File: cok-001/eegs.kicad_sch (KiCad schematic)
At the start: 54 parts, among them U7005 LM75B

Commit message: switching regulator
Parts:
- R7044, R7045: footprint Resistor_SMD:R_0603_1608Metric -> Resistor_SMD:R_0402_1005Metric
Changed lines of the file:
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@@
 			)
 		)
-		(property "Footprint" "Resistor_SMD:R_0603_1608Metric"
+		(property "Footprint" "Resistor_SMD:R_0402_1005Metric"
 			(at 555.244 141.224 90)
 			(effects
@@
 			)
 		)
-		(property "Footprint" "Resistor_SMD:R_0603_1608Metric"
+		(property "Footprint" "Resistor_SMD:R_0402_1005Metric"
 			(at 555.244 138.684 90)
 			(effects

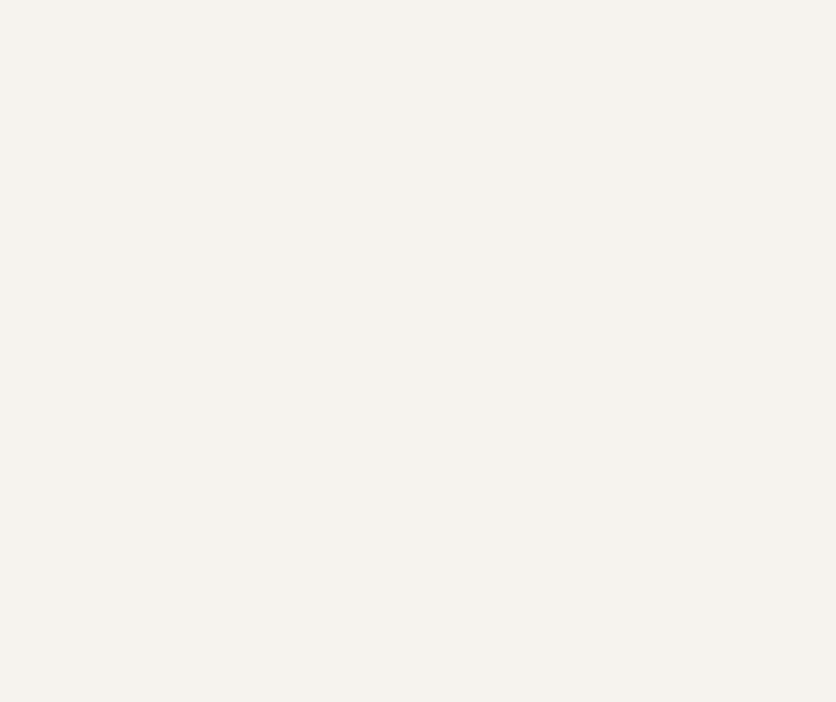
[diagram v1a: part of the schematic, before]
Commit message: temp sensor and clock
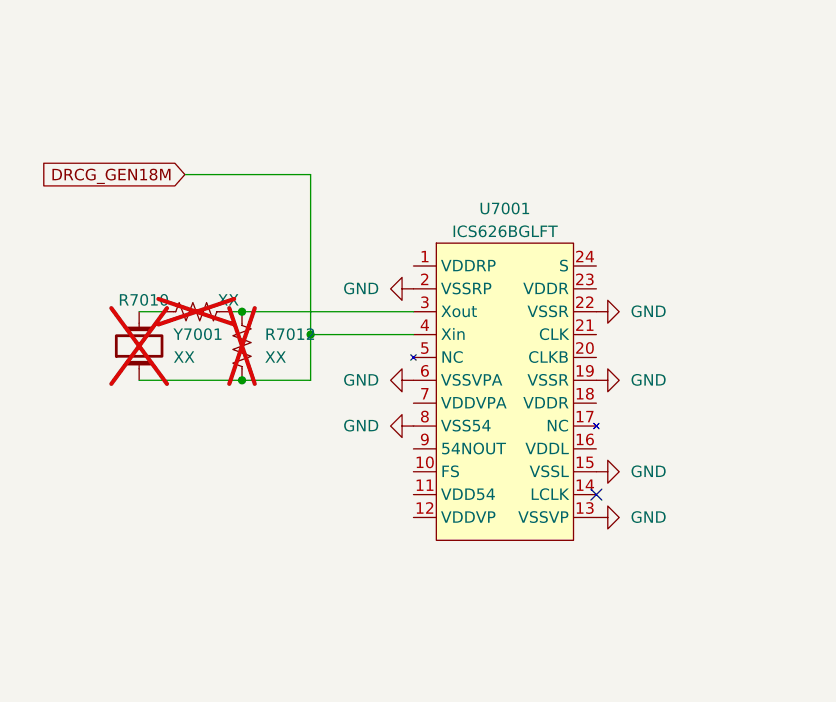
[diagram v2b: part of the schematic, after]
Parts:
- added R7010, R7012: XX, Resistor_SMD:R_0402_1005Metric, symbol Device:R_US
- added U7001: ICS626BGLFT, Package_SO:TSSOP-24_4.4x7.8mm_P0.65mm, symbol PS3:ICS626
- added Y7001: XX, Crystal:Crystal_SMD_FOX_FE-2Pin_7.5x5.0mm, symbol Device:Crystal
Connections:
- net GND: now also U7001.13 (VSSVP), U7001.15 (VSSL), U7001.19 (VSSR), U7001.2 (VSSRP), U7001.22 (VSSR), U7001.6 (VSSVPA), U7001.8 (VSS54)
- new net: R7010.2, R7012.2, U7001.3 (Xout)
- new net: R7010.1, Y7001.2
- new net DRCG_GEN18M: R7012.1, U7001.4 (Xin), Y7001.1
- no-connect marks 76 -> 77

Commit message: caps
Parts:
- added R7038: 22, Resistor_SMD:R_0402_1005Metric, symbol Device:R_US
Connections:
- net at U7004.A27 (SCK): now also R7038.1
- net at U7004.B27 (CMD): now also RN7021.3 (R3.1)
- net at RN7021.4 (R4.1): now also R7038.2
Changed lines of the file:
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@@
 	(wire
 		(pts
+			(xy 589.28 294.64) (xy 589.28 88.9)
+		)
+		(stroke
+			(width 0)
+			(type default)
+		)
+	)
+	(wire
+		(pts
 			(xy 458.47 -80.01) (xy 461.01 -80.01)
 		)
@@
 	(wire
 		(pts
+			(xy 229.87 289.56) (xy 586.74 289.56)
+		)
+		(stroke
+			(width 0)
+			(type default)
+		)
+	)
+	(wire
+		(pts
 			(xy 25.4 127) (xy 34.29 127)
 		)
@@
 	(wire
 		(pts
+			(xy 586.74 289.56) (xy 586.74 88.9)
+		)
+		(stroke
+			(width 0)
+			(type default)
+		)
+	)
+	(wire
+		(pts
 			(xy 538.48 -10.16) (xy 544.83 -10.16)
 		)
@@
 	(wire
 		(pts
+			(xy 227.33 294.64) (xy 236.22 294.64)
+		)
+		(stroke
+			(width 0)
+			(type default)
+		)
+	)
+	(wire
+		(pts
 			(xy 49.53 76.2) (xy 59.69 76.2)
 		)
@@
 	(wire
 		(pts
+			(xy 227.33 275.59) (xy 227.33 294.64)
+		)
+		(stroke
+			(width 0)
+			(type default)
+		)
+	)
+	(wire
+		(pts
 			(xy 232.41 275.59) (xy 234.95 275.59)
 		)
@@
 	(wire
 		(pts
+			(xy 229.87 275.59) (xy 229.87 289.56)
+		)
+		(stroke
+			(width 0)
+			(type default)
+		)
+	)
+	(wire
+		(pts
 			(xy 265.43 275.59) (xy 267.97 275.59)
 		)
@@
 	(wire
 		(pts
+			(xy 243.84 294.64) (xy 589.28 294.64)
+		)
+		(stroke
+			(width 0)
+			(type default)
+		)
+	)
+	(wire
+		(pts
 			(xy 106.68 170.18) (xy 106.68 172.72)
 		)
@@
 					(unit 1)
 				)
+			)
+		)
+	)
+	(symbol
+		(lib_id "Device:R_US")
+		(at 240.03 294.64 90)
+		(unit 1)
+		(exclude_from_sim no)
+		(in_bom yes)
+		(on_board yes)
+		(dnp no)
+		(property "Reference" "R7038"
+			(at 234.188 293.37 90)
+			(effects
+				(font
+					(size 1.27 1.27)
+				)
+			)
+		)
+		(property "Value" "22"
+			(at 243.586 293.37 90)
+			(effects
+				(font
+					(size 1.27 1.27)
+				)
+			)
+		)
+		(property "Footprint" "Resistor_SMD:R_0402_1005Metric"
+			(at 240.284 293.624 90)
+			(effects
+				(font
+					(size 1.27 1.27)
+				)
+				(hide yes)
+			)
+		)
+		(property "Datasheet" "~"
+			(at 240.03 294.64 0)
+			(effects
+				(font
+					(size 1.27 1.27)
+				)
+				(hide yes)
+			)
+		)
+		(property "Description" "Resistor, US symbol"
+			(at 240.03 294.64 0)
+			(effects
+				(font
+					(size 1.27 1.27)
+				)
+				(hide yes)
+			)
+		)
+		(pin "1"
+		)
+		(pin "2"
+		)
+		(instances
+			(project "cok-001"
+				(path "/976eb78d-8215-4cc0-9d72-f9d535c7970b/83bad906-8af5-42c9-8580-60b7c8083ecb"
+					(reference "R7038")
+					(unit 1)
+				)
